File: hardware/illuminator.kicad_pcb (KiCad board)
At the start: 4 copper layers, 85 x 100 mm, 63 parts, among them J101 HRO_TYPE_C_31_M_12, J102 PROG, J103 LCLV, Q201 DMP3028, Q202 MMBT3904, SW101 RESET, SW102 DFU, U101 SRV05-4, U102 STM32G431CBUx, U103 WAS3157B-6/TR, U104 TL072, U105 HT7550-1_C16106, U106 78L05G-AB3-R, Y101 12MHz

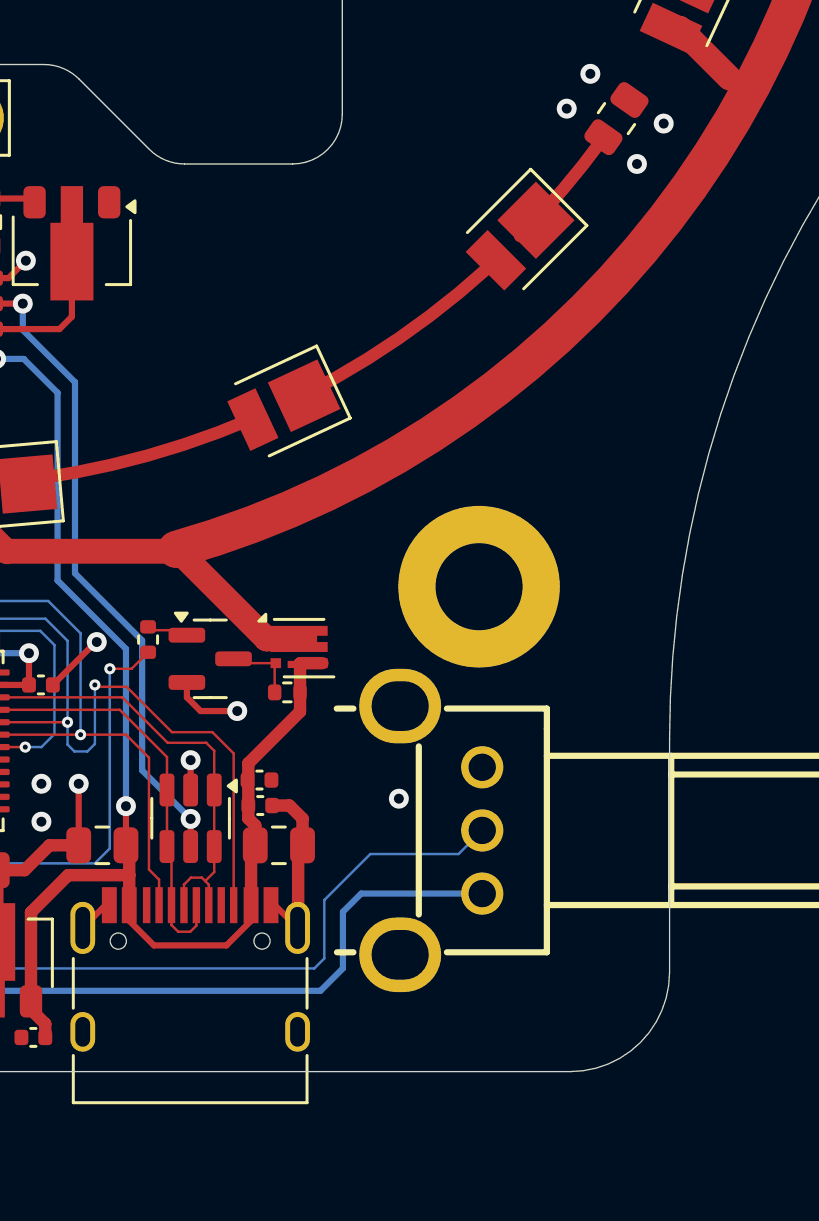
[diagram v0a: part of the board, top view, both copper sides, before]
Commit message: fix bom
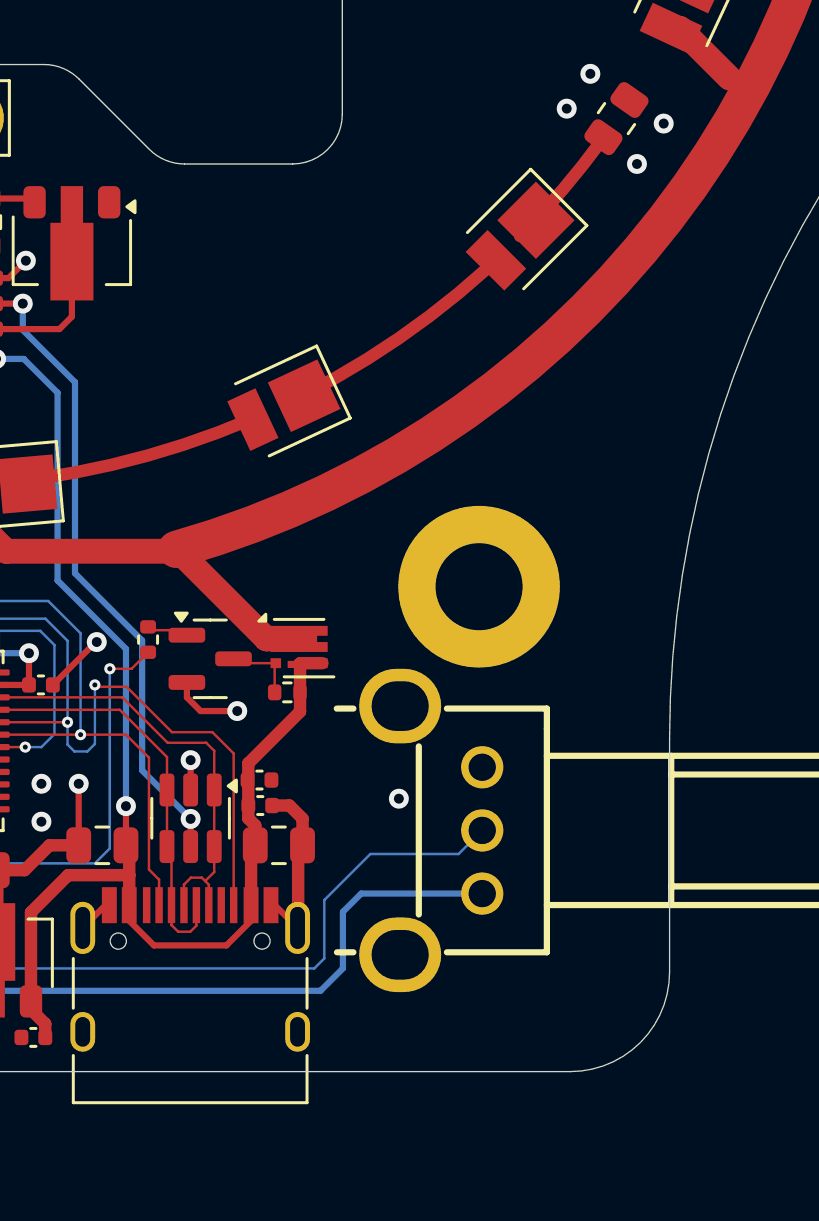
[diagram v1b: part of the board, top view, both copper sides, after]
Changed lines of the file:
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@@
 			(viasonmask no)
 			(mode 1)
-			(useauxorigin no)
+			(useauxorigin yes)
 			(hpglpennumber 1)
 			(hpglpenspeed 20)
@@
 			(outputformat 1)
 			(mirror no)
-			(drillshape 1)
+			(drillshape 0)
 			(scaleselection 1)
-			(outputdirectory "")
+			(outputdirectory "/Users/mateijordache/Desktop/gerbs/")
 		)
 	)
@@
 		(fp_arc
 			(start 10.656836 20.999983)
-			(mid 9.891468 20.847747)
+			(mid 9.891462 20.847753)
 			(end 9.242623 20.414196)
 			(stroke
@@
 		(fp_arc
 			(start 30.160875 53.5)
-			(mid 28.989302 56.328425)
+			(mid 28.989302 56.328429)
 			(end 26.160875 57.5)
 			(stroke
